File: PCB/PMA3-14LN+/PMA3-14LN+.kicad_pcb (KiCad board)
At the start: 4 copper layers, 55.3 x 35 mm, 26 parts, among them U1 PMA3-14LN+, U2 L7806

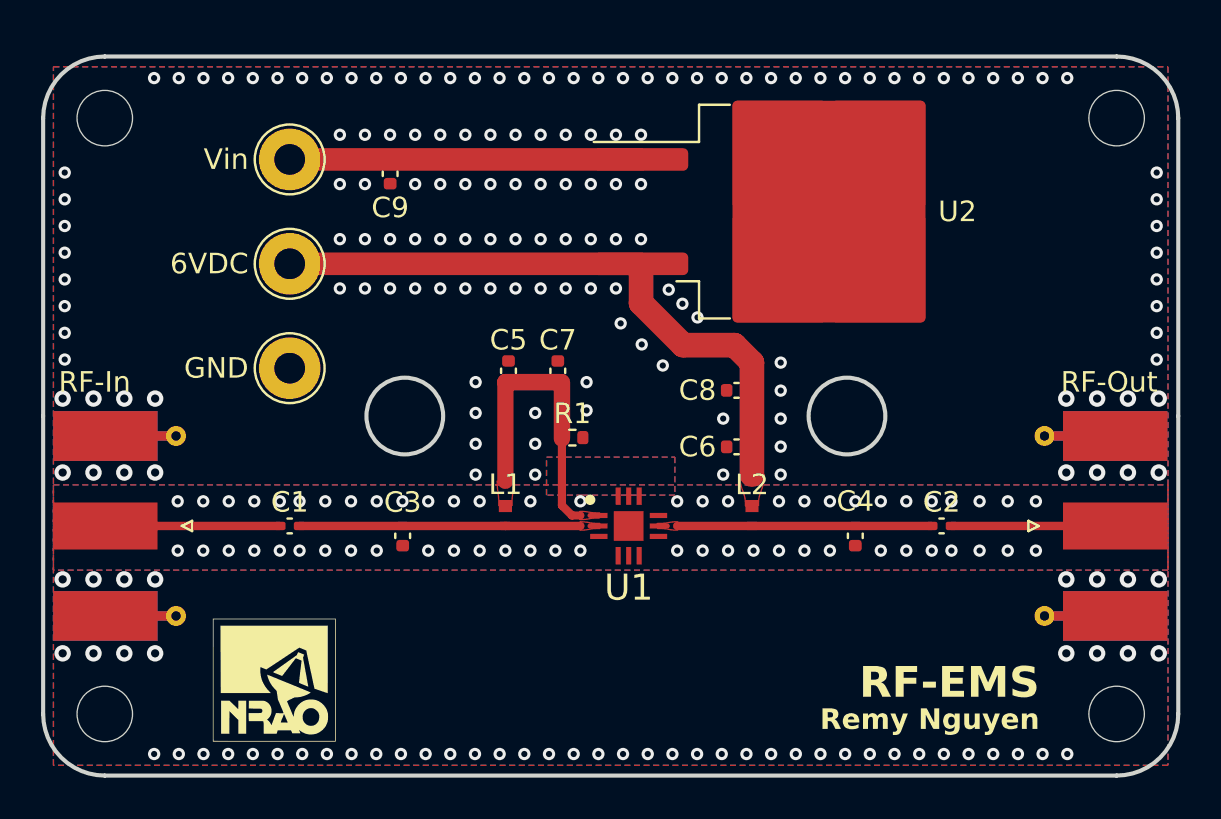
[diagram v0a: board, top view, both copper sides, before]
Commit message: PMA3-14LN+ Rev B Complete
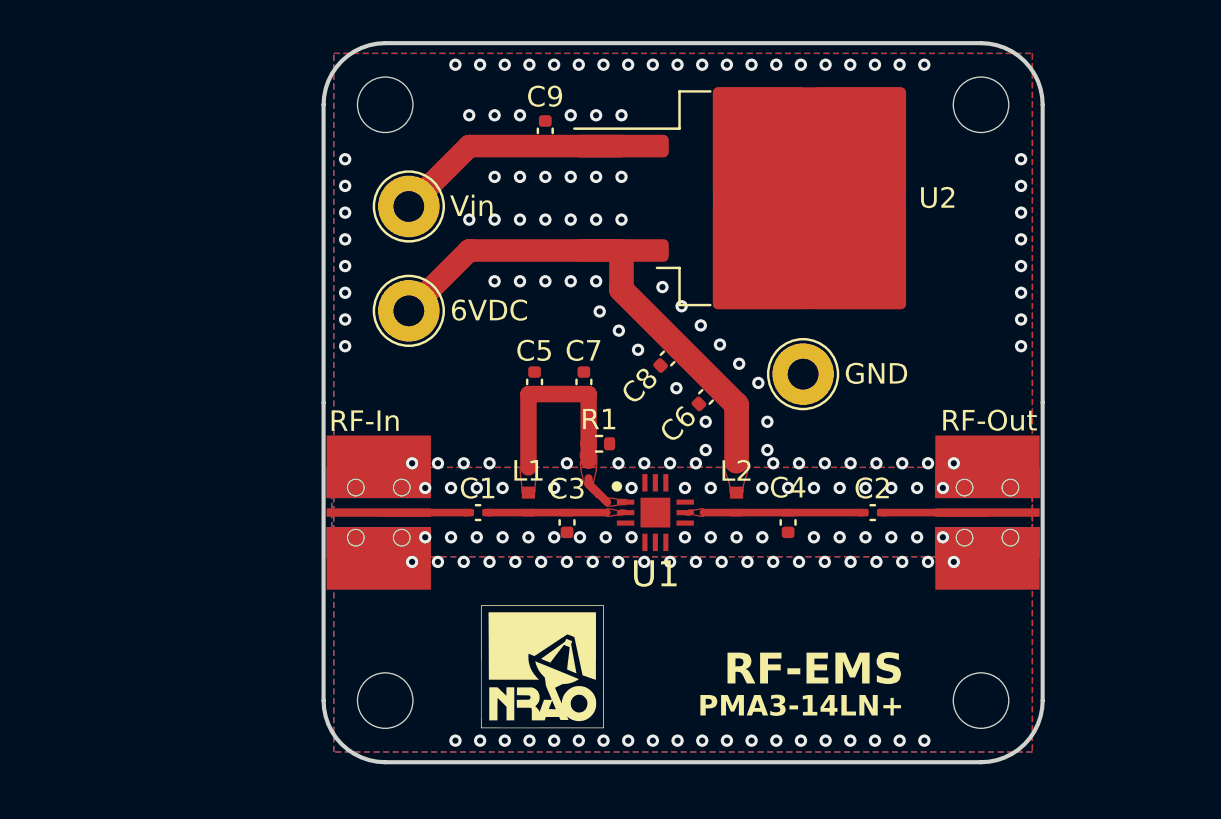
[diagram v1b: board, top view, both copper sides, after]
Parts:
- removed ?: , imports:RF-DFS-GCPW-OSH
- added REF**: LOGO, rf-dfs:GCPW_osh3_90mm_user, F.Cu at (207.0, 147.5)
- RF-In, RF-Out: footprint footprints:SMA_Molex_73251-1153_EdgeMount_Horizontal_TunedOSH -> rf-dfs:Mueller BU-1420761881-RevB
- moved GND 25.0 mm to (147.8, 86.6)
- moved REF** 13.7 mm to (127.5, 73.5)
- moved REF** 13.7 mm to (127.5, 102.5)
- moved RF-In 13.5 mm to (129.0, 93.3)
- moved G*** 13.1 mm to (135.2, 100.8)
- moved C1 9.19 mm to (132.0, 93.3)
- moved C3 8.03 mm to (136.3, 93.8)
- moved C9 7.83 mm to (135.3, 74.8), turned to 90 degrees
- moved REF** 6.63 mm to (156.5, 102.5)
- moved REF** 6.63 mm to (156.5, 73.5)
- moved RF-Out 6.38 mm to (155.0, 93.3)
- moved 6VDC 6.24 mm to (128.7, 83.5)
- moved Vin 6.24 mm to (128.7, 78.5)
- moved C8 3.70 mm to (141.2, 85.8), turned to -135 degrees
- moved C2 3.41 mm to (151.2, 93.3)
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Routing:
- net Net-(IC1-RF-IN): track 14.1 -> 5.79 mm
- net 6VDC: track 30.5 -> 23.6 mm
- net Vin: track 17.1 -> 11.6 mm
- net Net-(IC1-RF-OUT_&_VDD): track 12.8 -> 7.76 mm
- net Net-(J1-In): track 8.70 -> 4.35 mm
- net Net-(IC1-CURRENT_MIRROR): track 15.0 -> 11.3 mm
- net Net-(J2-In): track 8.22 -> 5.10 mm
- net GND: vias 255 -> 168
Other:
- board size 55.3 x 35 mm -> 35 x 35 mm
- board text added: "10/24/2024"
- board text added: "B"
- board text added: "Rev B"
- board text removed: "4/12/2024"
- board text removed: "A"
- board text removed: "Hole pattern for Hammond 1554B"
